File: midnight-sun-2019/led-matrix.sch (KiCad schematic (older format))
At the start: 476 parts

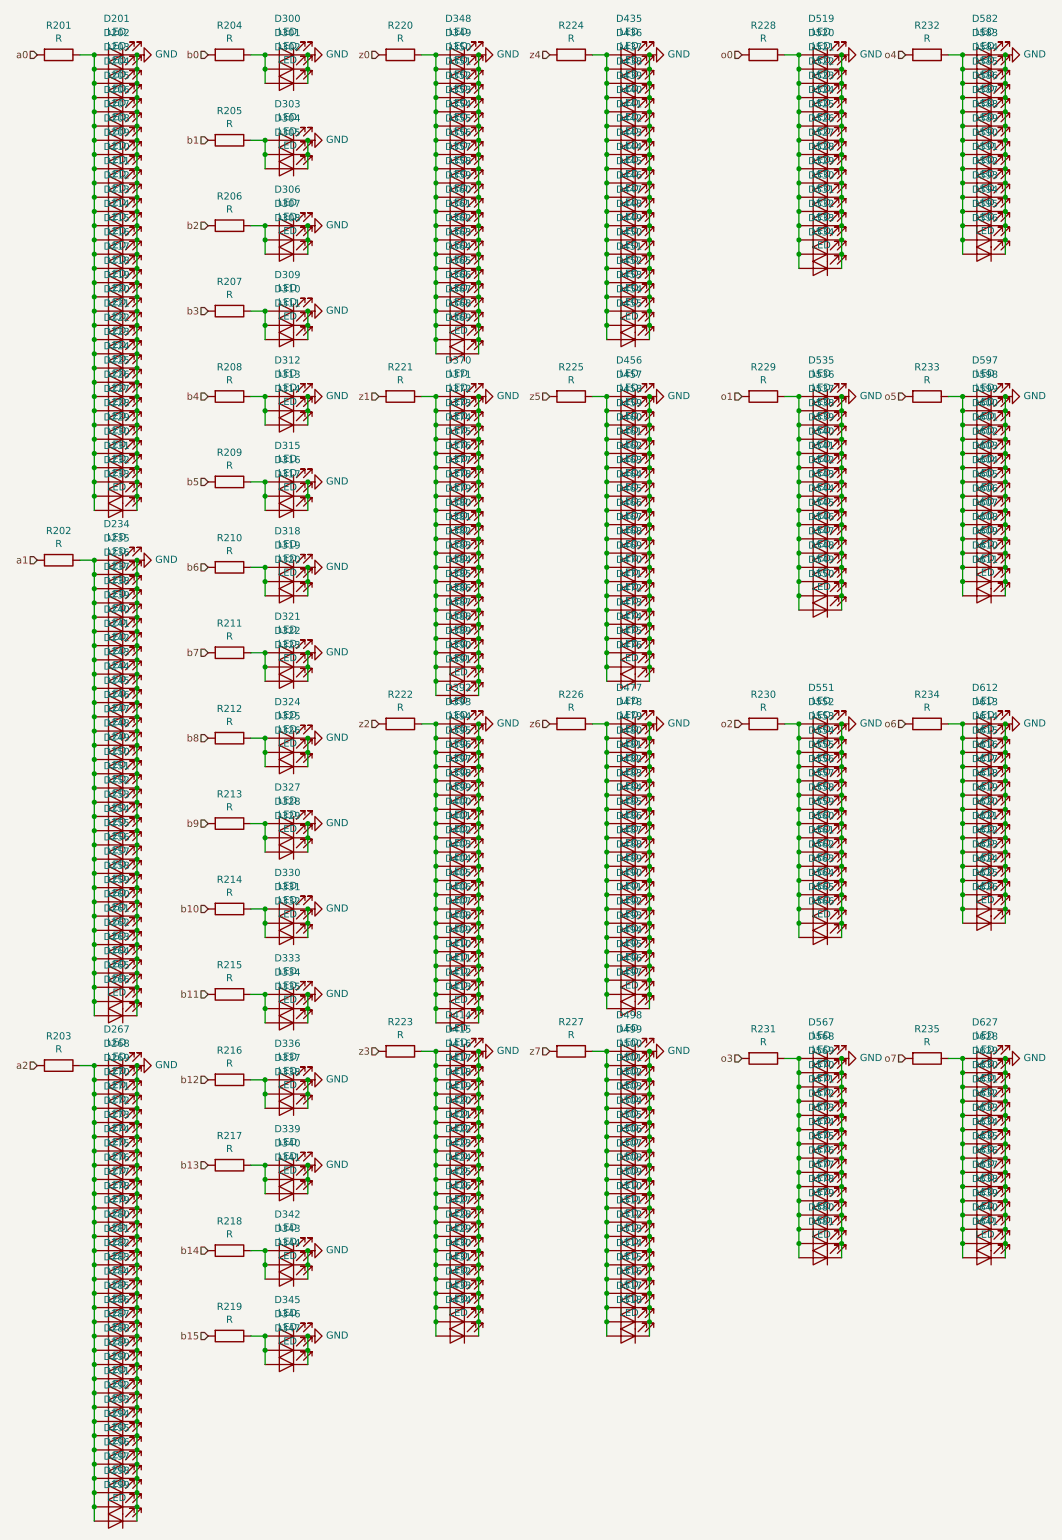
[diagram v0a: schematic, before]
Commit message: Re-annotate components
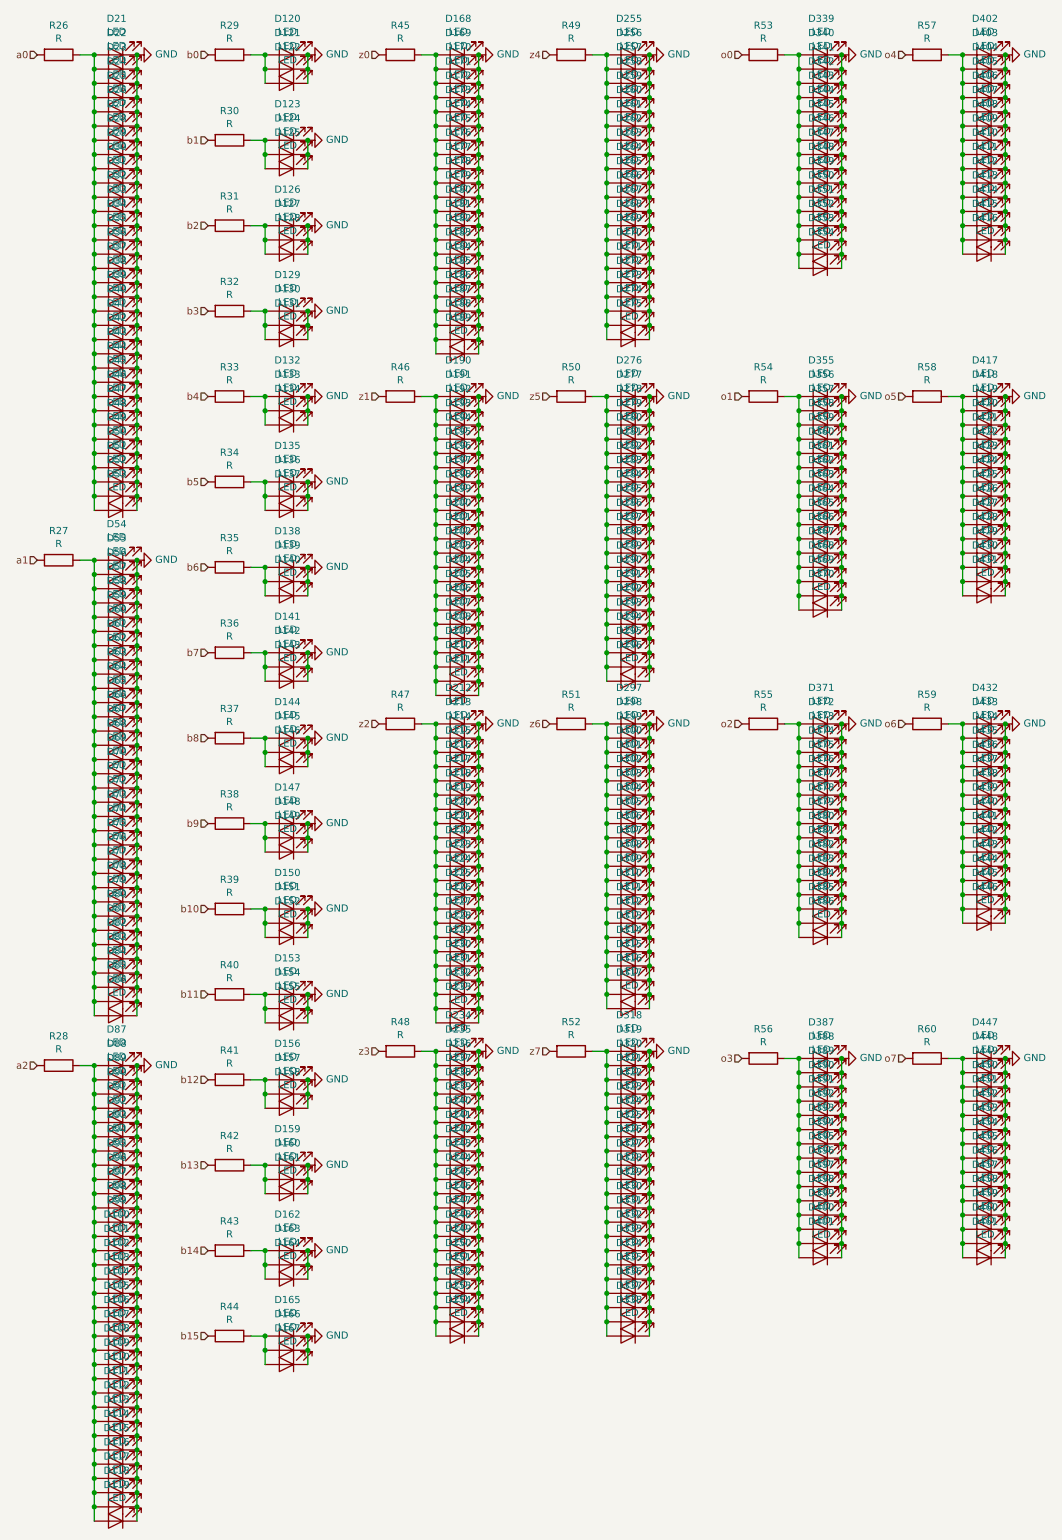
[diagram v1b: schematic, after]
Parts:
- renumbered D280 to D100, D281 to D101, D282 to D102, D283 to D103, D284 to D104, D285 to D105, D286 to D106, D287 to D107, D288 to D108, D289 to D109, D290 to D110, D291 to D111, D292 to D112, D293 to D113, D294 to D114, D295 to D115, D296 to D116, D297 to D117, D298 to D118, D299 to D119, D300 to D120, D301 to D121, D302 to D122, D303 to D123, D304 to D124, D305 to D125, D306 to D126, D307 to D127, D308 to D128, D309 to D129, D310 to D130, D311 to D131, D312 to D132, D313 to D133, D314 to D134, D315 to D135, D316 to D136, D317 to D137, D318 to D138, D319 to D139, D320 to D140, D321 to D141, D322 to D142, D323 to D143, D324 to D144, D325 to D145, D326 to D146, D327 to D147, D328 to D148, D329 to D149, D330 to D150, D331 to D151, D332 to D152, D333 to D153, D334 to D154, D335 to D155, D336 to D156, D337 to D157, D338 to D158, D339 to D159, D340 to D160, D341 to D161, D342 to D162, D343 to D163, D344 to D164, D345 to D165, D346 to D166, D347 to D167, D348 to D168, D349 to D169, D350 to D170, D351 to D171, D352 to D172, D353 to D173, D354 to D174, D355 to D175, D356 to D176, D357 to D177, D358 to D178, D359 to D179, D360 to D180, D361 to D181, D362 to D182, D363 to D183, D364 to D184, D365 to D185, D366 to D186, D367 to D187, D368 to D188, D369 to D189, D370 to D190, D371 to D191, D372 to D192, D373 to D193, D374 to D194, D375 to D195, D376 to D196, D377 to D197, D378 to D198, D379 to D199, D380 to D200, D381 to D201, D382 to D202, D383 to D203, D384 to D204, D385 to D205, D386 to D206, D387 to D207, D388 to D208, D389 to D209, D201 to D21, D390 to D210, D391 to D211, D392 to D212, D393 to D213, D394 to D214, D395 to D215, D396 to D216, D397 to D217, D398 to D218, D399 to D219, D202 to D22, D400 to D220, D401 to D221, D402 to D222, D403 to D223, D404 to D224, D405 to D225, D406 to D226, D407 to D227, D408 to D228, D409 to D229, D203 to D23, D410 to D230, D411 to D231, D412 to D232, D413 to D233, D414 to D234, D415 to D235, D416 to D236, D417 to D237, D418 to D238, D419 to D239, D204 to D24, D420 to D240, D421 to D241, D422 to D242, D423 to D243, D424 to D244, D425 to D245, D426 to D246, D427 to D247, D428 to D248, D429 to D249, D205 to D25, D430 to D250, D431 to D251, D432 to D252, D433 to D253, D434 to D254, D435 to D255, D436 to D256, D437 to D257, D438 to D258, D439 to D259, D206 to D26, D440 to D260, D441 to D261, D442 to D262, D443 to D263, D444 to D264, D445 to D265, D446 to D266, D447 to D267, D448 to D268, D449 to D269, D207 to D27, D450 to D270, D451 to D271, D452 to D272, D453 to D273, D454 to D274, D455 to D275, D456 to D276, D457 to D277, D458 to D278, D459 to D279, D208 to D28, D460 to D280, D461 to D281, D462 to D282, D463 to D283, D464 to D284, D465 to D285, D466 to D286, D467 to D287, D468 to D288, D469 to D289, D209 to D29, D470 to D290, D471 to D291, D472 to D292, D473 to D293, D474 to D294, D475 to D295, D476 to D296, D477 to D297, D478 to D298, D479 to D299, D210 to D30, D480 to D300, D481 to D301, D482 to D302, D483 to D303, D484 to D304, D485 to D305, D486 to D306, D487 to D307, D488 to D308, D489 to D309, D211 to D31, D490 to D310, D491 to D311, D492 to D312, D493 to D313, D494 to D314, D495 to D315, D496 to D316, D497 to D317, D498 to D318, D499 to D319, D212 to D32, D500 to D320, D501 to D321, D502 to D322, D503 to D323, D504 to D324, D505 to D325, D506 to D326, D507 to D327, D508 to D328, D509 to D329, D213 to D33, D510 to D330, D511 to D331, D512 to D332, D513 to D333, D514 to D334, D515 to D335, D516 to D336, D517 to D337, D518 to D338, D519 to D339, D214 to D34, D520 to D340, D521 to D341, D522 to D342, D523 to D343, D524 to D344, D525 to D345, D526 to D346, D527 to D347, D528 to D348, D529 to D349, D215 to D35, D530 to D350, D531 to D351, D532 to D352, D533 to D353, D534 to D354, D535 to D355, D536 to D356, D537 to D357, D538 to D358, D539 to D359, D216 to D36, D540 to D360, D541 to D361, D542 to D362, D543 to D363, D544 to D364, D545 to D365, D546 to D366, D547 to D367, D548 to D368, D549 to D369, D217 to D37, D550 to D370, D551 to D371, D552 to D372, D553 to D373, D554 to D374, D555 to D375, D556 to D376, D557 to D377, D558 to D378, D559 to D379, D218 to D38, D560 to D380, D561 to D381, D562 to D382, D563 to D383, D564 to D384, D565 to D385, D566 to D386, D567 to D387, D568 to D388, D569 to D389, D219 to D39, D570 to D390, D571 to D391, D572 to D392, D573 to D393, D574 to D394, D575 to D395, D576 to D396, D577 to D397, D578 to D398, D579 to D399, D220 to D40, D580 to D400, D581 to D401, D582 to D402, D583 to D403, D584 to D404, D585 to D405, D586 to D406, D587 to D407, D588 to D408, D589 to D409, D221 to D41, D590 to D410, D591 to D411, D592 to D412, D593 to D413, D594 to D414, D595 to D415, D596 to D416, D597 to D417, D598 to D418, D599 to D419, D222 to D42, D600 to D420, D601 to D421, D602 to D422, D603 to D423, D604 to D424, D605 to D425, D606 to D426, D607 to D427, D608 to D428, D609 to D429, D223 to D43, D610 to D430, D611 to D431, D612 to D432, D613 to D433, D614 to D434, D615 to D435, D616 to D436, D617 to D437, D618 to D438, D619 to D439, D224 to D44, D620 to D440, D621 to D441, D622 to D442, D623 to D443, D624 to D444, D625 to D445, D626 to D446, D627 to D447, D628 to D448, D629 to D449, D225 to D45, D630 to D450, D631 to D451, D632 to D452, D633 to D453, D634 to D454, D635 to D455, D636 to D456, D637 to D457, D638 to D458, D639 to D459, D226 to D46, D640 to D460, D641 to D461, D227 to D47, D228 to D48, D229 to D49, D230 to D50, D231 to D51, D232 to D52, D233 to D53, D234 to D54, D235 to D55, D236 to D56, D237 to D57, D238 to D58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

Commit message: More finishing touches
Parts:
- D21, D22, D23, D24, D25: footprint LED_SMD:LED_0805_2012Metric_Castellated -> electrokit:LED_0805_2012Metric_Castellated_no_silkscreen
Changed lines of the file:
@@
 F 0 "D22" H 1193 645 50  0000 C CNN
 F 1 "LED" H 1193 736 50  0000 C CNN
-F 2 "LED_SMD:LED_0805_2012Metric_Castellated" H 1200 900 50  0001 C CNN
+F 2 "electrokit:LED_0805_2012Metric_Castellated_no_silkscreen" H 1200 900 50  0001 C CNN
 F 3 "~" H 1200 900 50  0001 C CNN
 	1    1200 900
@@
 F 0 "D24" H 1193 845 50  0000 C CNN
 F 1 "LED" H 1193 936 50  0000 C CNN
-F 2 "LED_SMD:LED_0805_2012Metric_Castellated" H 1200 1100 50  0001 C CNN
+F 2 "electrokit:LED_0805_2012Metric_Castellated_no_silkscreen" H 1200 1100 50  0001 C CNN
 F 3 "~" H 1200 1100 50  0001 C CNN
 	1    1200 1100
@@
 F 0 "D25" H 1193 945 50  0000 C CNN
 F 1 "LED" H 1193 1036 50  0000 C CNN
-F 2 "LED_SMD:LED_0805_2012Metric_Castellated" H 1200 1200 50  0001 C CNN
+F 2 "electrokit:LED_0805_2012Metric_Castellated_no_silkscreen" H 1200 1200 50  0001 C CNN
 F 3 "~" H 1200 1200 50  0001 C CNN
 	1    1200 1200
@@
 F 0 "D23" H 1193 745 50  0000 C CNN
 F 1 "LED" H 1193 836 50  0000 C CNN
-F 2 "LED_SMD:LED_0805_2012Metric_Castellated" H 1200 1000 50  0001 C CNN
+F 2 "electrokit:LED_0805_2012Metric_Castellated_no_silkscreen" H 1200 1000 50  0001 C CNN
 F 3 "~" H 1200 1000 50  0001 C CNN
 	1    1200 1000
@@
 F 0 "D21" H 1193 545 50  0000 C CNN
 F 1 "LED" H 1193 636 50  0000 C CNN
-F 2 "LED_SMD:LED_0805_2012Metric_Castellated" H 1200 800 50  0001 C CNN
+F 2 "electrokit:LED_0805_2012Metric_Castellated_no_silkscreen" H 1200 800 50  0001 C CNN
 F 3 "~" H 1200 800 50  0001 C CNN
 	1    1200 800

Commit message: More finishing touches
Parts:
- D100, D101, D102, D103, D104, D105, D106, D107, D108, D109, D110, D111, D112, D113, D114, D115, D116, D117, D118, D119, D120, D121, D122, D123, D124, D125, D126, D127, D128, D129, D130, D131, D132, D133, D134, D135, D136, D137, D138, D139, D140, D141, D142, D143, D144, D145, D146, D147, D148, D149, D150, D151, D152, D153, D154, D155, D156, D157, D158, D159, D160, D161, D162, D163, D164, D165, D166, D167, D168, D169, D170, D171, D172, D173, D174, D175, D176, D177, D178, D179, D180, D181, D182, D183, D184, D185, D186, D187, D188, D189, D190, D191, D192, D193, D194, D195, D196, D197, D198, D199, D200, D201, D202, D203, D204, D205, D206, D207, D208, D209, D210, D211, D212, D213, D214, D215, D216, D217, D218, D219, D220, D221, D222, D223, D224, D225, D226, D227, D228, D229, D230, D231, D232, D233, D234, D235, D236, D237, D238, D239, D240, D241, D242, D243, D244, D245, D246, D247, D248, D249, D250, D251, D252, D253, D254, D255, D256, D257, D258, D259, D26, D260, D261, D262, D263, D264, D265, D266, D267, D268, D269, D27, D270, D271, D272, D273, D274, D275, D276, D277, D278, D279, D28, D280, D281, D282, D283, D284, D285, D286, D287, D288, D289, D29, D290, D291, D292, D293, D294, D295, D296, D297, D298, D299, D30, D300, D301, D302, D303, D304, D305, D306, D307, D308, D309, D31, D310, D311, D312, D313, D314, D315, D316, D317, D318, D319, D32, D320, D321, D322, D323, D324, D325, D326, D327, D328, D329, D33, D330, D331, D332, D333, D334, D335, D336, D337, D338, D339, D34, D340, D341, D342, D343, D344, D345, D346, D347, D348, D349, D35, D350, D351, D352, D353, D354, D355, D356, D357, D358, D359, D36, D360, D361, D362, D363, D364, D365, D366, D367, D368, D369, D37, D370, D371, D372, D373, D374, D375, D376, D377, D378, D379, D38, D380, D381, D382, D383, D384, D385, D386, D387, D388, D389, D39, D390, D391, D392, D393, D394, D395, D396, D397, D398, D399, D40, D400, D401, D402, D403, D404, D405, D406, D407, D408, D409, D41, D410, D411, D412, D413, D414, D415, D416, D417, D418, D419, D42, D420, D421, D422, D423, D424, D425, D426, D427, D428, D429, D43, D430, D431, D432, D433, D434, D435, D436, D437, D438, D439, D44, D440, D441, D442, D443, D444, D445, D446, D447, D448, D449, D45, D450, D451, D452, D453, D454, D455, D456, D457, D458, D459, D46, D460, D461, D47, D48, D49, D50, D51, D52, D53, D54, D55, D56, D57, D58, D59, D60, D61, D62, D63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: footprint LED_SMD:LED_0805_2012Metric_Castellated -> electrokit:LED_0805_2012Metric_Castellated_no_silkscreen
